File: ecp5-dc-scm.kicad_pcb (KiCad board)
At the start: 8 copper layers, 90 x 120.4 mm, 458 parts, among them IC1 TPS54561, J1 L834-1G1T-S7, J2 1-2199230-6, J3 529910408, J4 M20-7830642, J5 SFF-TA-1002-4C+, J6 0878311420, J7 61300611121, J8 S2B-PH-K-S_LF__SN_, Q1 2N7002, Q10 2N7002, Q11 2N7002, Q12 2N7002, Q13 2N7002, Q14 2N7002, Q15 2N7002, Q16 2N7002, Q17 2N7002, Q2 2N7002, Q3 2N7002, U1 KSZ9031RNXCA, U10 AS4C256M16D3, U11 TPS51200DRC, U12 LM3881MME_NOPB, U13 LM21212-2, U14 AMJMEFB-100.0000T, U16 TPS62823DLCT, U17 TPS62823DLCT, U18 TPS62823DLCT, U19 TPS62823DLCT, U2 W25Q32JVSSIQ_TR, U20 TPS62823DLCT, U21 ECP5UM5G_85_CABGA756, U3 W25Q32JVSSIQ_TR, U4 W25Q32JVSSIQ_TR, U5 W25Q32JVSSIQ_TR, U6 MTFC32GAPALBH-AIT, U7 NVT2008DQ,115, U8 USB3300-EZK-TR, U9 USB3300-EZK-TR, Y1 ABM8G-25.000MHZ-18-D2Y-T, Y2 TSX-3225, Y3 TSX-3225

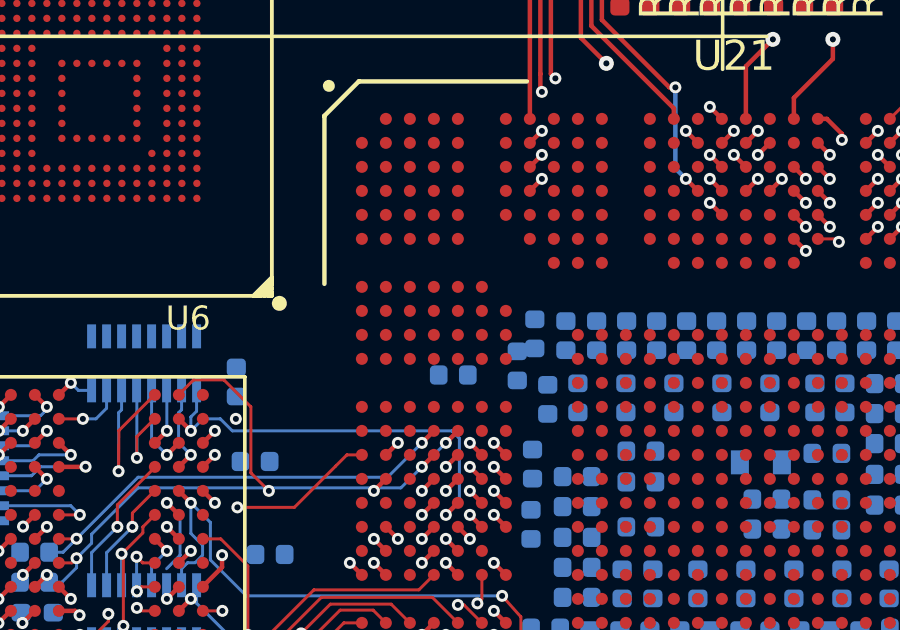
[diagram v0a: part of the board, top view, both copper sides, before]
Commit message: Started sketching MMC
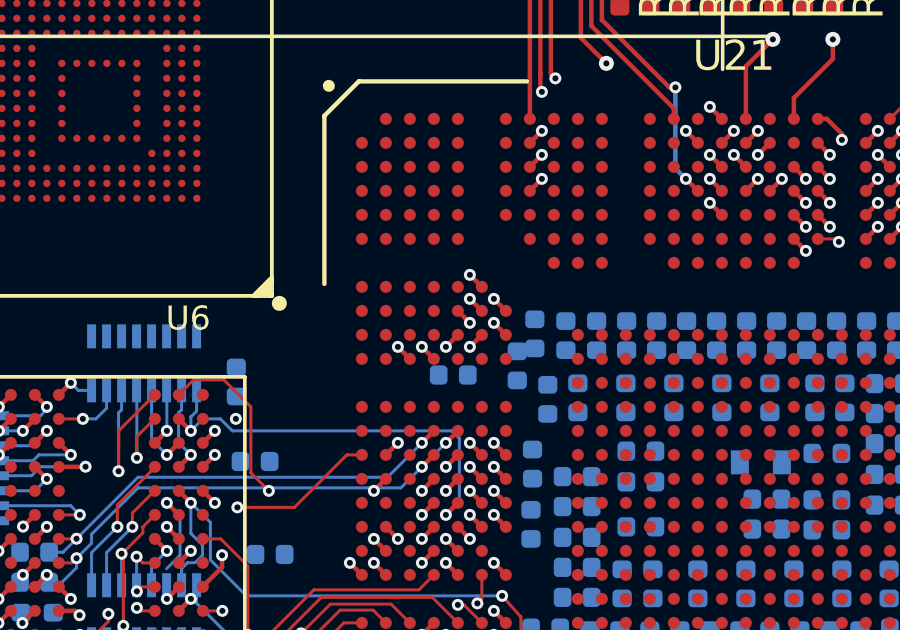
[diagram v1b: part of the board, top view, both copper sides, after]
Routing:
- net MMC_CMD: track 0.00 -> 15.4 mm, vias 0 -> 1
- net MMC_CLK: track 0.00 -> 14.6 mm, vias 0 -> 2
- net MMC_DAT6: track 0.00 -> 14.1 mm, vias 0 -> 1
- net MMC_DAT7: track 0.00 -> 13.5 mm, vias 0 -> 1
- net MMC_DAT4: track 0.00 -> 12.3 mm, vias 0 -> 1
- net MMC_DAT5: track 0.00 -> 12.2 mm, vias 0 -> 1
- net MMC_DAT3: track 0.00 -> 10.4 mm, vias 0 -> 1
- net GND: track 108.0 -> 108.6 mm, vias 95 -> 96
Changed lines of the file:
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@@
     (thickness 1.57)
     (drawings 80)
-    (tracks 3757)
+    (tracks 3801)
     (zones 0)
     (modules 458)
@@
   (segment (start 59 114.514256) (end 39.435744 94.95) (width 0.1) (layer F.Cu) (net 0))
   (segment (start 59 115.05) (end 59 114.514256) (width 0.1) (layer F.Cu) (net 0))
+  (via (at 95.6 114.95) (size 0.4) (drill 0.2) (layers F.Cu B.Cu) (net 1))
+  (segment (start 95.2 114.55) (end 95.6 114.95) (width 0.15) (layer F.Cu) (net 1))
+  (via (at 95.6 113.35) (size 0.4) (drill 0.2) (layers F.Cu B.Cu) (net 356))
+  (segment (start 96 113.75) (end 95.6 113.35) (width 0.15) (layer F.Cu) (net 356))
+  (via (at 95.6 114.15) (size 0.4) (drill 0.2) (layers F.Cu B.Cu) (net 354))
+  (segment (start 96 114.55) (end 95.6 114.15) (width 0.15) (layer F.Cu) (net 354))
+  (via (at 96.4 114.15) (size 0.4) (drill 0.2) (layers F.Cu B.Cu) (net 355))
+  (segment (start 96.8 114.55) (end 96.4 114.15) (width 0.15) (layer F.Cu) (net 355))
+  (via (at 96.4 114.95) (size 0.4) (drill 0.2) (layers F.Cu B.Cu) (net 351))
+  (segment (start 96.8 115.35) (end 96.4 114.95) (width 0.15) (layer F.Cu) (net 351))
+  (via (at 95.6 115.75) (size 0.4) (drill 0.2) (layers F.Cu B.Cu) (net 353))
+  (segment (start 96 115.35) (end 95.6 115.75) (width 0.15) (layer F.Cu) (net 353))
+  (via (at 94.8 115.75) (size 0.4) (drill 0.2) (layers F.Cu B.Cu) (net 352))
+  (segment (start 95.2 115.35) (end 94.8 115.75) (width 0.15) (layer F.Cu) (net 352))
+  (via (at 94 115.75) (size 0.4) (drill 0.2) (layers F.Cu B.Cu) (net 350))
+  (segment (start 94.4 116.15) (end 94 115.75) (width 0.15) (layer F.Cu) (net 350))
+  (via (at 93.2 115.75) (size 0.4) (drill 0.2) (layers F.Cu B.Cu) (net 356))
+  (segment (start 93.6 116.15) (end 93.2 115.75) (width 0.15) (layer F.Cu) (net 356))
   (via (at 109.2 109.35) (size 0.4) (drill 0.2) (layers F.Cu B.Cu) (net 45))
   (segment (start 109.6 109.75) (end 109.2 109.35) (width 0.15) (layer F.Cu) (net 45))
@@
   (via (at 113.25 155.3) (size 0.5) (drill 0.2) (layers F.Cu B.Cu) (net 328))
   (via (at 113.85 153.65) (size 0.5) (drill 0.2) (layers F.Cu B.Cu) (net 330))
+  (segment (start 94 115.75) (end 93.55 115.3) (width 0.1) (layer In2.Cu) (net 350))
+  (segment (start 93.55 115.3) (end 90.55 115.3) (width 0.1) (layer In2.Cu) (net 350))
+  (segment (start 90.55 115.3) (end 86.25 111) (width 0.1) (layer In2.Cu) (net 350))
+  (segment (start 86.25 111) (end 86.2 110.95) (width 0.1) (layer In2.Cu) (net 350))
+  (segment (start 90.2 114.55) (end 86.65 111) (width 0.1) (layer In2.Cu) (net 351))
+  (segment (start 96.4 114.95) (end 96 115.35) (width 0.1) (layer In2.Cu) (net 351))
+  (segment (start 94.35 115.35) (end 93.55 114.55) (width 0.1) (layer In2.Cu) (net 351))
+  (segment (start 96 115.35) (end 94.35 115.35) (width 0.1) (layer In2.Cu) (net 351))
+  (segment (start 93.55 114.55) (end 90.2 114.55) (width 0.1) (layer In2.Cu) (net 351))
+  (segment (start 94.8 115.75) (end 94.8 115.8) (width 0.1) (layer In2.Cu) (net 352))
+  (segment (start 94.8 115.8) (end 94.45 116.15) (width 0.1) (layer In2.Cu) (net 352))
+  (segment (start 94.45 116.15) (end 90.9 116.15) (width 0.1) (layer In2.Cu) (net 352))
+  (segment (start 90.9 116.15) (end 85.6 110.85) (width 0.1) (layer In2.Cu) (net 352))
+  (segment (start 90.65 116.4) (end 84.8 110.55) (width 0.1) (layer In2.Cu) (net 353))
+  (segment (start 95.6 115.75) (end 94.95 116.4) (width 0.1) (layer In2.Cu) (net 353))
+  (segment (start 94.95 116.4) (end 90.65 116.4) (width 0.1) (layer In2.Cu) (net 353))
+  (segment (start 95.6 114.15) (end 90.65 114.15) (width 0.1) (layer In2.Cu) (net 354))
+  (segment (start 90.65 114.15) (end 86.55 110.05) (width 0.1) (layer In2.Cu) (net 354))
+  (segment (start 86.55 110.05) (end 84.35 110.05) (width 0.1) (layer In2.Cu) (net 354))
+  (segment (start 96.4 114.15) (end 96.35 114.1) (width 0.1) (layer In2.Cu) (net 355))
+  (segment (start 96.35 114.1) (end 96.35 113.45) (width 0.1) (layer In2.Cu) (net 355))
+  (segment (start 96.35 113.45) (end 95.8 112.9) (width 0.1) (layer In2.Cu) (net 355))
+  (segment (start 95.8 112.9) (end 91.3 112.9) (width 0.1) (layer In2.Cu) (net 355))
+  (segment (start 91.3 112.9) (end 85.05 106.65) (width 0.1) (layer In2.Cu) (net 355))
+  (segment (start 95.6 113.35) (end 91.35 113.35) (width 0.1) (layer In2.Cu) (net 356))
+  (segment (start 91.35 113.35) (end 84.85 106.85) (width 0.1) (layer In2.Cu) (net 356))
   (zone (net 0) (net_name "") (layers F.Cu GND1 In2.Cu VCC1 GND2 B.Cu) (hatch edge 0.508)
     (connect_pads (clearance 0.508))
